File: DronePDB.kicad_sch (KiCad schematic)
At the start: 8 parts

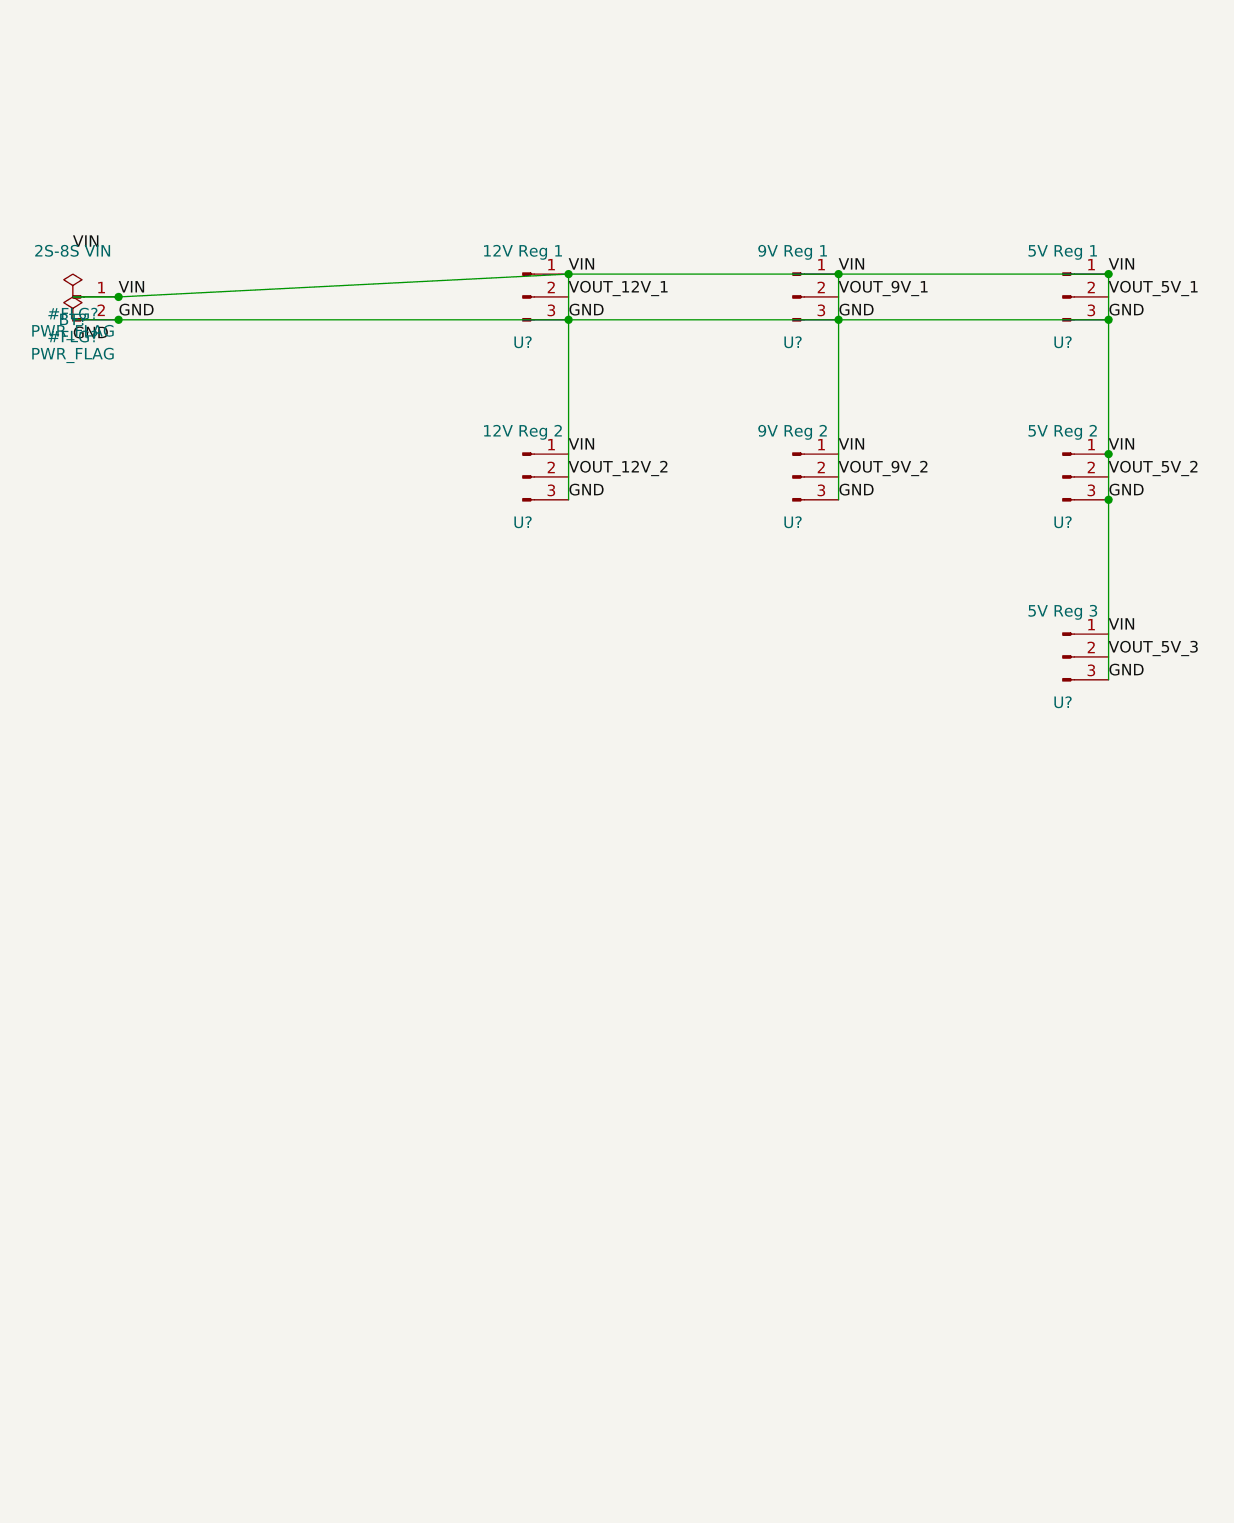
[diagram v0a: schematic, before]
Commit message: update
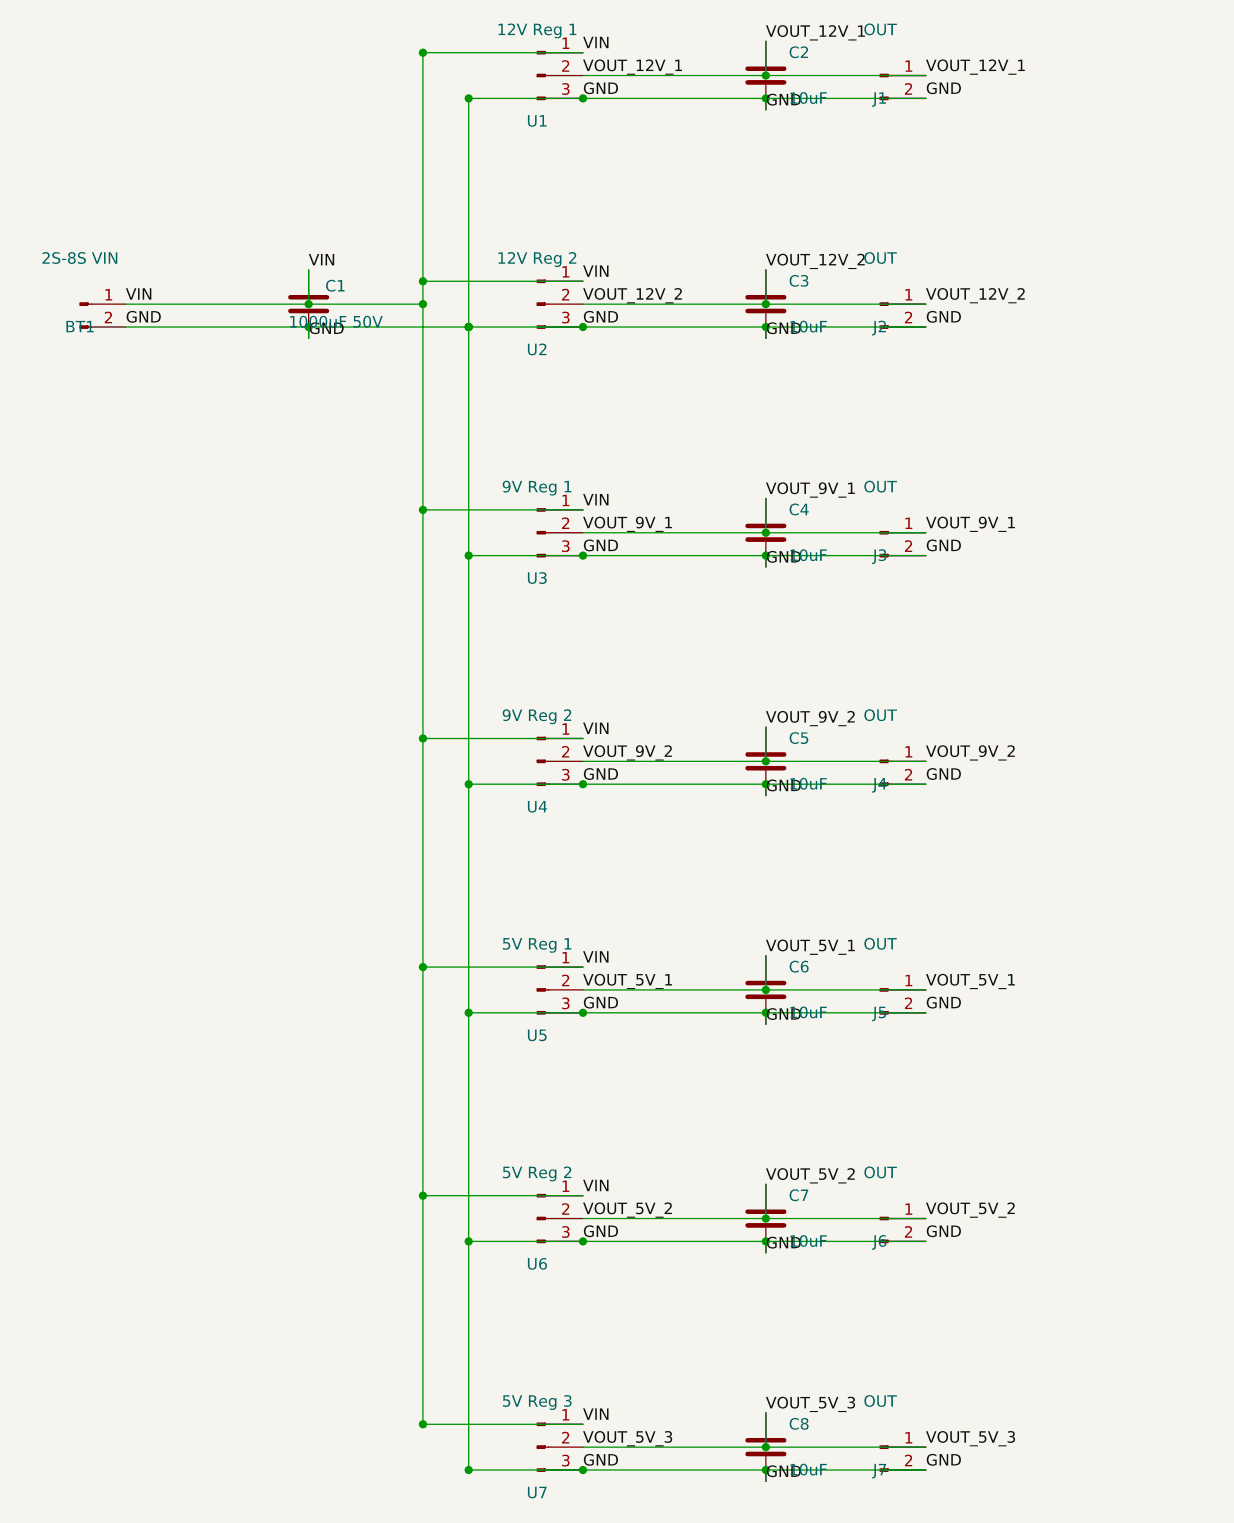
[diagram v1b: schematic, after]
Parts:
- removed BT?: 2S-8S VIN, Connector_AMASS:AMASS_XT60-M_1x02_P7.20mm_Vertical, symbol Connector:Conn_01x02_Pin
- removed U?: 12V Reg 2, Connector_PinHeader_2.54mm:PinHeader_1x03_P2.54mm_Vertical, symbol Connector:Conn_01x03_Pin
- removed U?: 9V Reg 2, Connector_PinHeader_2.54mm:PinHeader_1x03_P2.54mm_Vertical, symbol Connector:Conn_01x03_Pin
- removed U?: 12V Reg 1, Connector_PinHeader_2.54mm:PinHeader_1x03_P2.54mm_Vertical, symbol Connector:Conn_01x03_Pin
- removed U?: 5V Reg 2, Connector_PinHeader_2.54mm:PinHeader_1x03_P2.54mm_Vertical, symbol Connector:Conn_01x03_Pin
- removed U?: 5V Reg 1, Connector_PinHeader_2.54mm:PinHeader_1x03_P2.54mm_Vertical, symbol Connector:Conn_01x03_Pin
- removed U?: 5V Reg 3, Connector_PinHeader_2.54mm:PinHeader_1x03_P2.54mm_Vertical, symbol Connector:Conn_01x03_Pin
- removed U?: 9V Reg 1, Connector_PinHeader_2.54mm:PinHeader_1x03_P2.54mm_Vertical, symbol Connector:Conn_01x03_Pin
- added BT1: 2S-8S VIN, Connector_AMASS:AMASS_XT60-M_1x02_P7.20mm_Vertical, symbol Connector:Conn_01x02_Pin
- added C1: 1000uF 50V, Capacitor_THT:CP_Radial_D8.0mm_P3.50mm, symbol Device:C
- added C2, C3, C4, C5, C6, C7, C8: 10uF, Capacitor_SMD:C_0805_2012Metric, symbol Device:C
- added J1, J2, J3, J4, J5, J6, J7: OUT, Connector_PinHeader_2.54mm:PinHeader_1x02_P2.54mm_Vertical, symbol Connector:Conn_01x02_Pin
- added U1: 12V Reg 1, Connector_PinHeader_2.54mm:PinHeader_1x03_P2.54mm_Vertical, symbol Connector:Conn_01x03_Pin
- added U2: 12V Reg 2, Connector_PinHeader_2.54mm:PinHeader_1x03_P2.54mm_Vertical, symbol Connector:Conn_01x03_Pin
- added U3: 9V Reg 1, Connector_PinHeader_2.54mm:PinHeader_1x03_P2.54mm_Vertical, symbol Connector:Conn_01x03_Pin
- added U4: 9V Reg 2, Connector_PinHeader_2.54mm:PinHeader_1x03_P2.54mm_Vertical, symbol Connector:Conn_01x03_Pin
- added U5: 5V Reg 1, Connector_PinHeader_2.54mm:PinHeader_1x03_P2.54mm_Vertical, symbol Connector:Conn_01x03_Pin
- added U6: 5V Reg 2, Connector_PinHeader_2.54mm:PinHeader_1x03_P2.54mm_Vertical, symbol Connector:Conn_01x03_Pin
- added U7: 5V Reg 3, Connector_PinHeader_2.54mm:PinHeader_1x03_P2.54mm_Vertical, symbol Connector:Conn_01x03_Pin
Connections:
- net GND: now also BT1.2 (Pin_2), C1.2, C2.2, C3.2, C4.2, C5.2, C6.2, C7.2, C8.2, J1.2 (Pin_2), J2.2 (Pin_2), J3.2 (Pin_2), J4.2 (Pin_2), J5.2 (Pin_2), J6.2 (Pin_2), J7.2 (Pin_2), U1.3 (Pin_3), U2.3 (Pin_3), U3.3 (Pin_3), U4.3 (Pin_3), U5.3 (Pin_3), U6.3 (Pin_3), U7.3 (Pin_3)
- new net VIN: BT1.1 (Pin_1), C1.1, U1.1 (Pin_1), U2.1 (Pin_1), U3.1 (Pin_1), U4.1 (Pin_1), U5.1 (Pin_1), U6.1 (Pin_1), U7.1 (Pin_1)
- new net VOUT_12V_1: C2.1, J1.1 (Pin_1), U1.2 (Pin_2)
- new net VOUT_12V_2: C3.1, J2.1 (Pin_1), U2.2 (Pin_2)
- new net VOUT_5V_1: C6.1, J5.1 (Pin_1), U5.2 (Pin_2)
- new net VOUT_5V_2: C7.1, J6.1 (Pin_1), U6.2 (Pin_2)
- new net VOUT_5V_3: C8.1, J7.1 (Pin_1), U7.2 (Pin_2)
- new net VOUT_9V_1: C4.1, J3.1 (Pin_1), U3.2 (Pin_2)
- new net VOUT_9V_2: C5.1, J4.1 (Pin_1), U4.2 (Pin_2)
